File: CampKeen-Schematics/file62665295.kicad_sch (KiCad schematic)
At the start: 32 parts, among them Q2 2N7000, Q3 IRF9Z34NPBF, Q4 2N7000, Q5 2N7000, Q58 LTV-847, Q6 2N7000, Q7 2N7000

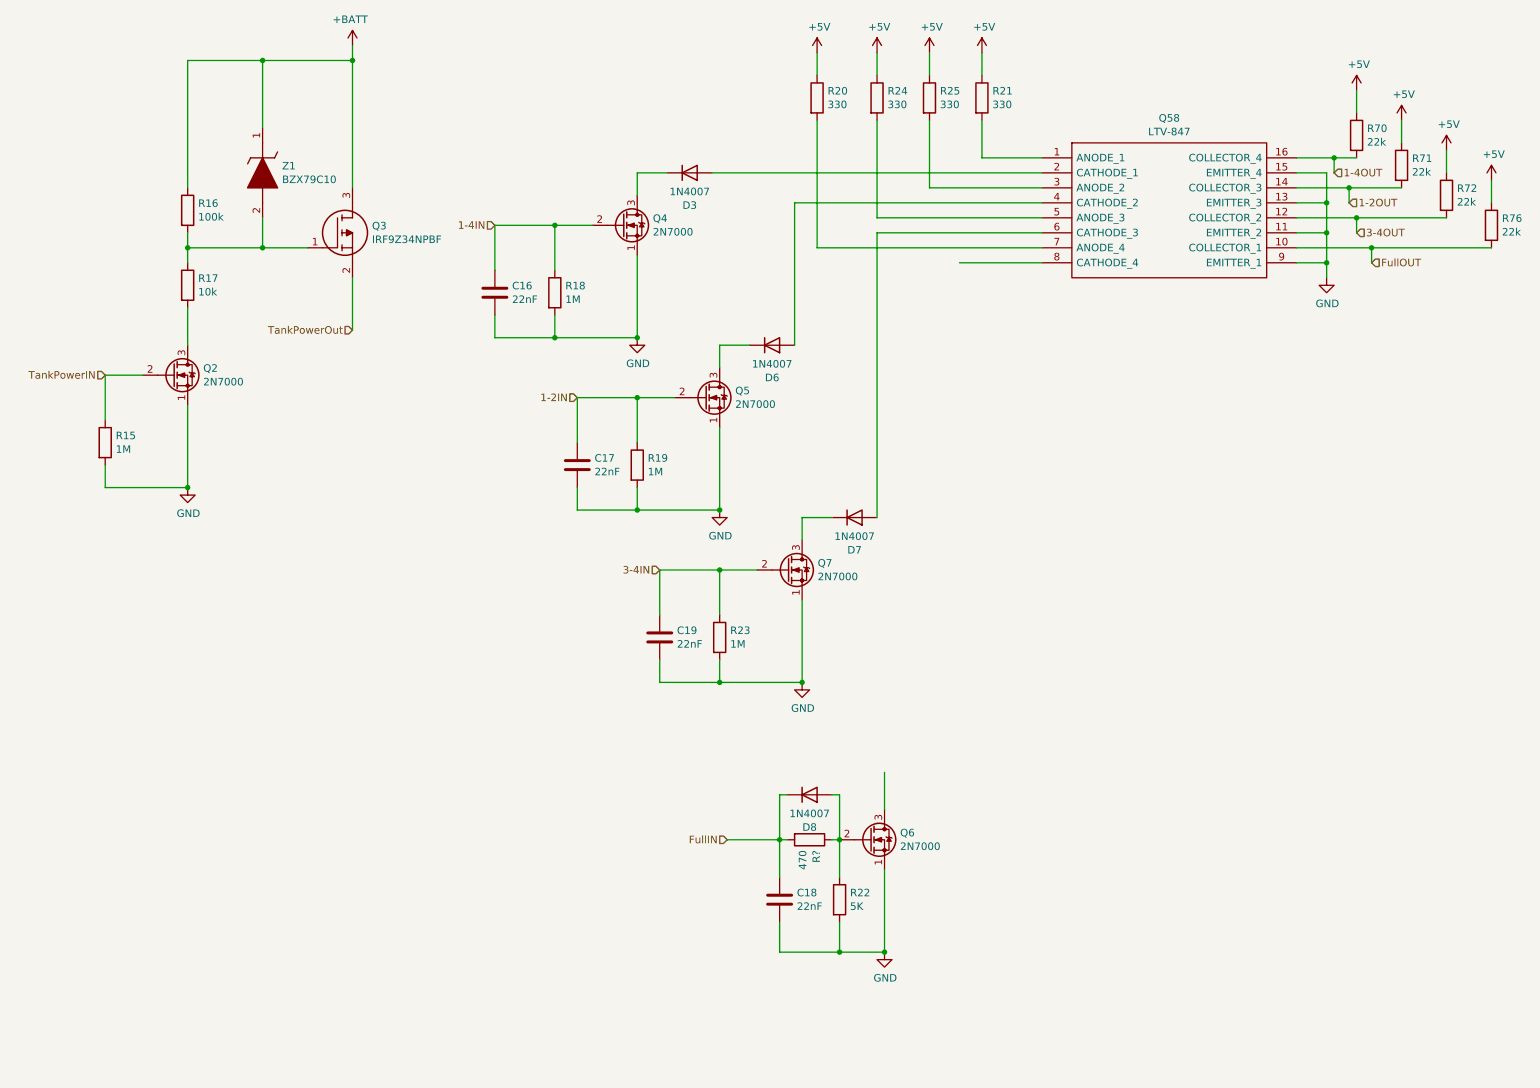
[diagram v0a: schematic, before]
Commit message: wip removing the traces fixing the inputs
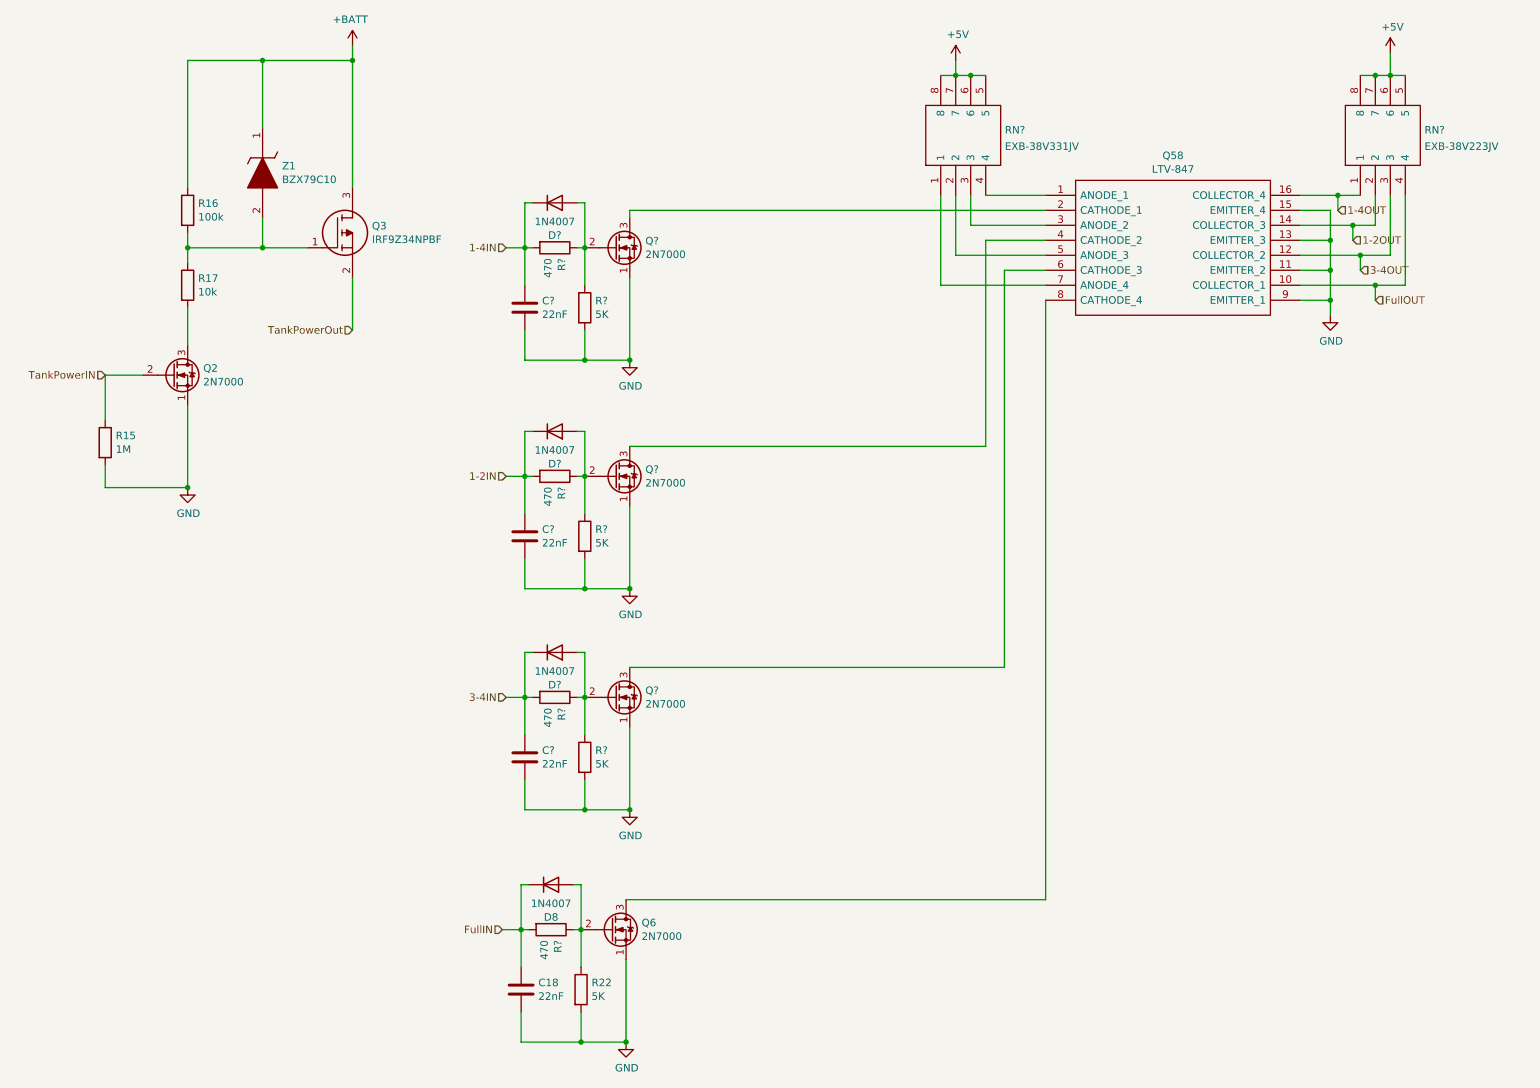
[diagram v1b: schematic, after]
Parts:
- removed C16, C17, C19: 22nF, Capacitor_THT:C_Disc_D4.7mm_W2.5mm_P5.00mm, symbol Device:C
- removed D3, D6, D7: 1N4007, Diode_THT:D_DO-41_SOD81_P10.16mm_Horizontal, symbol Diode:1N4007
- removed Q4, Q5, Q7: 2N7000, Package_TO_SOT_THT:TO-92_Inline, symbol Transistor_FET:2N7000
- removed R18, R19, R23: 1M, Resistor_THT:R_Axial_DIN0207_L6.3mm_D2.5mm_P2.54mm_Vertical, symbol Device:R
- removed R20, R21, R24, R25: 330, Resistor_THT:R_Axial_DIN0207_L6.3mm_D2.5mm_P2.54mm_Vertical, symbol Device:R
- removed R70, R71, R72, R76: 22k, Resistor_THT:R_Axial_DIN0207_L6.3mm_D2.5mm_P2.54mm_Vertical, symbol Device:R
- added C? (x3): 22nF, Capacitor_THT:C_Disc_D4.7mm_W2.5mm_P5.00mm, symbol Device:C
- added D? (x3): 1N4007, Diode_THT:D_DO-41_SOD81_P10.16mm_Horizontal, symbol Diode:1N4007
- added Q? (x3): 2N7000, Package_TO_SOT_THT:TO-92_Inline, symbol Transistor_FET:2N7000
- added R? (x3): 5K, Resistor_THT:R_Axial_DIN0207_L6.3mm_D2.5mm_P2.54mm_Vertical, symbol Device:R
- added R? (x3): 470, Resistor_THT:R_Axial_DIN0207_L6.3mm_D2.5mm_P2.54mm_Vertical, symbol Device:R
- added RN?: EXB-38V331JV, EXB38V472JV, symbol Samac_Sys:EXB-38V331JV
- added RN?: EXB-38V223JV, EXB38V472JV, symbol Samac_Sys:EXB-38V223JV
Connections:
- net +5V: now also RN?.5, RN?.5, RN?.6, RN?.6, RN?.7, RN?.7, RN?.8, RN?.8
- net 1-2IN: now also C?.1, D?.1 (K), R?.2
- net 1-2OUT: now also RN?.2
- net 1-4IN: now also C?.1, D?.1 (K), R?.2
- net 1-4OUT: now also RN?.1
- net 3-4IN: now also C?.1, D?.1 (K), R?.2
- net 3-4OUT: now also RN?.3
- net FullOUT: now also RN?.4
- net GND: now also C?.2, C?.2, C?.2, Q?.1 (S), Q?.1 (S), Q?.1 (S), R?.2, R?.2, R?.2
- net at Q58.2 (CATHODE_1): now also Q?.3 (D)
- net at Q58.4 (CATHODE_2): now also Q?.3 (D)
- net at Q58.6 (CATHODE_3): now also Q?.3 (D)
- net at Q58.1 (ANODE_1): now also RN?.4
- net at Q58.3 (ANODE_2): now also RN?.3
- net at Q58.5 (ANODE_3): now also RN?.2
- net at Q58.7 (ANODE_4): now also RN?.1
- net at Q58.8 (CATHODE_4): now also Q6.3 (D)
- new net: D?.2 (A), Q?.2 (G), R?.1, R?.1 (x3)
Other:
- moved on the sheet: C18, D8, Q58, Q6, R22, R?
